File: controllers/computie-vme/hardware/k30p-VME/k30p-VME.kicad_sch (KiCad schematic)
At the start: 8 parts, among them J1 5V, J2 5V

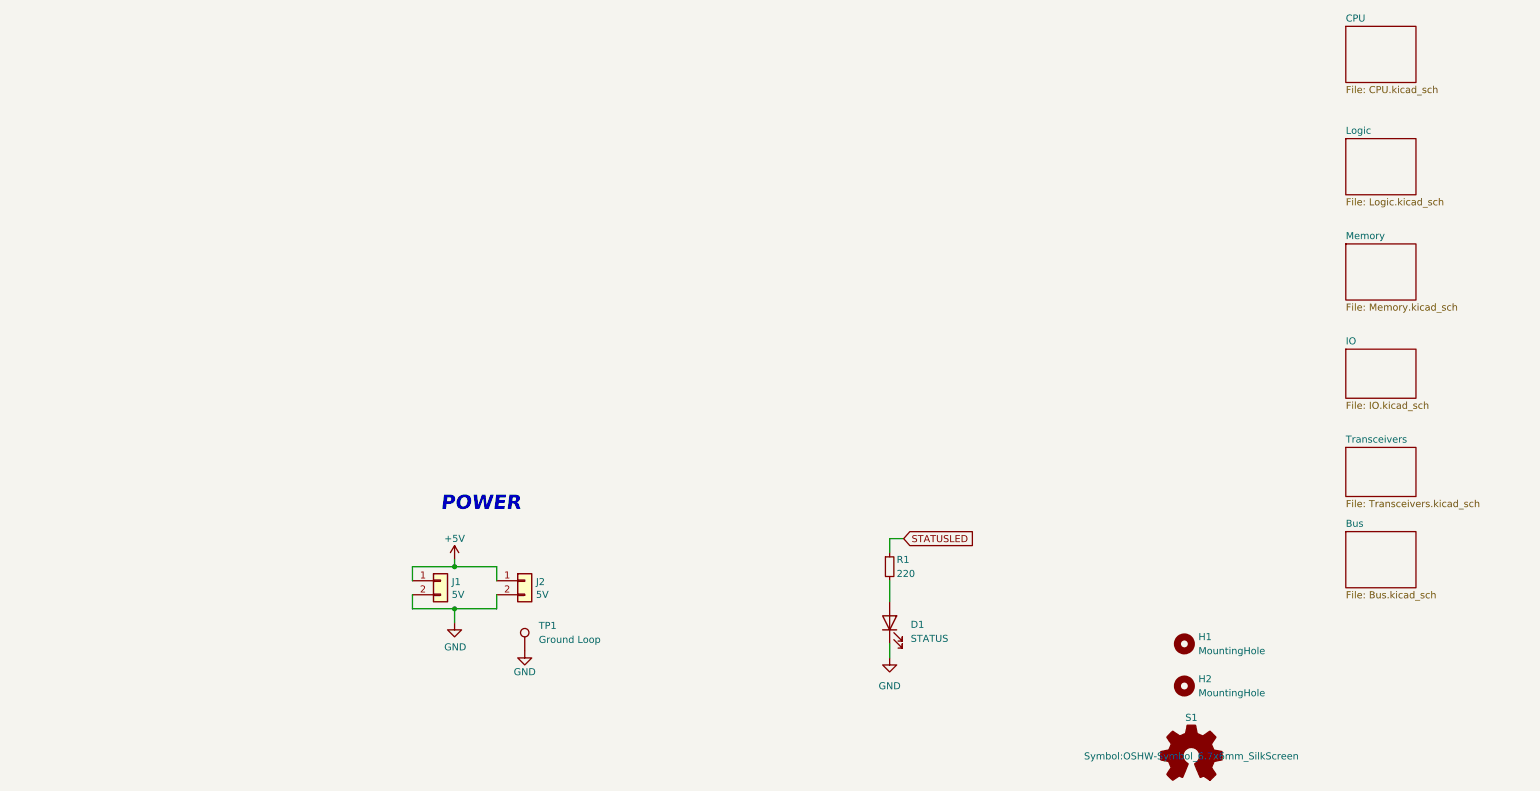
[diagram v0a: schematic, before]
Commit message: Updating with more work in progress
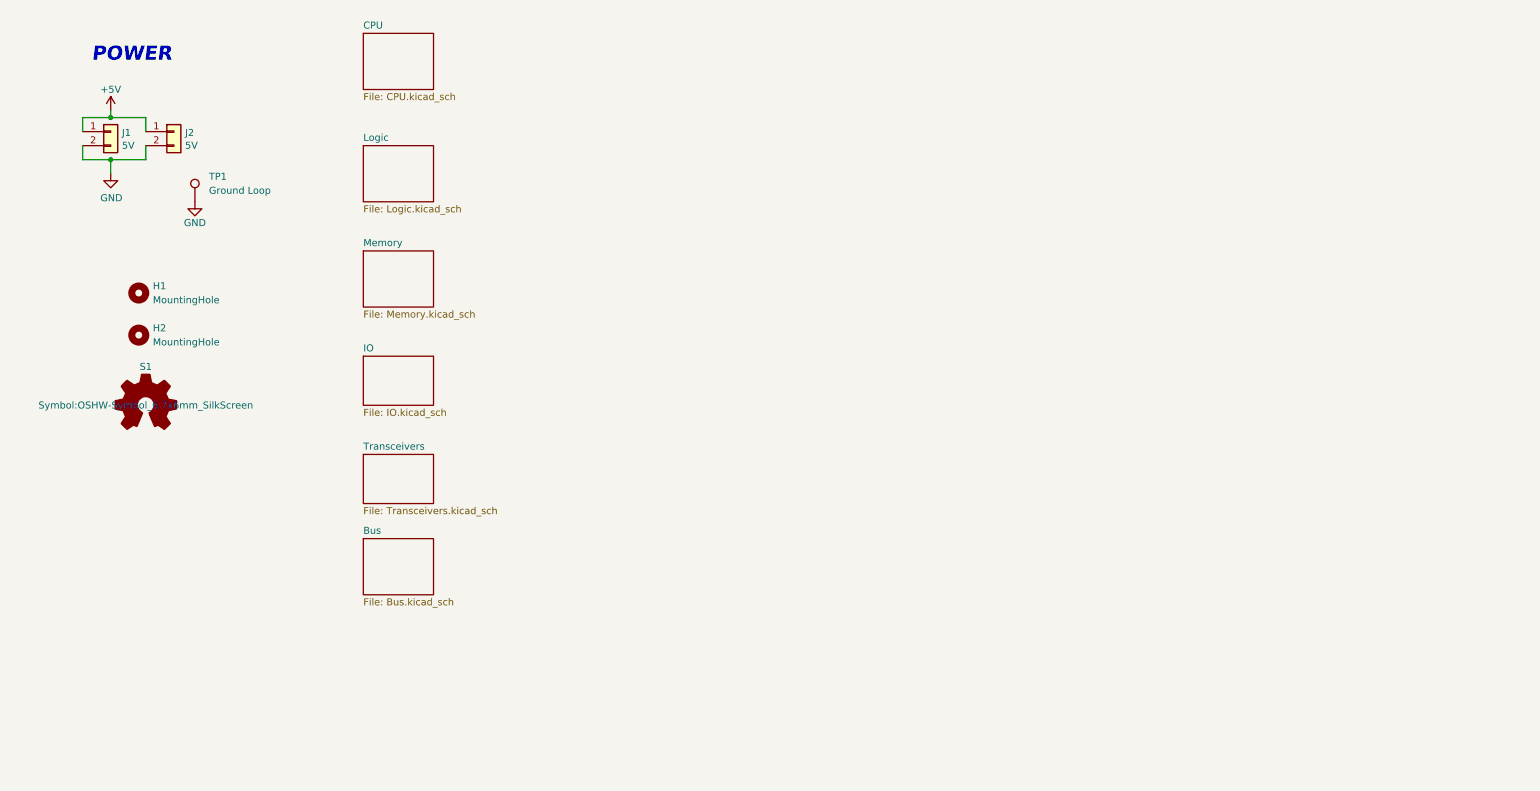
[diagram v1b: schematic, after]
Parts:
- removed D1: STATUS, LED_THT:LED_D3.0mm, symbol Device:LED
- removed R1: 220, Resistor_SMD:R_0805_2012Metric_Pad1.20x1.40mm_HandSolder, symbol Device:R_Small
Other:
- title: k30-VME32 -> k30p-VME
- moved on the sheet: H1, H2, J1, J2, S1, TP1

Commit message: Reorganized a bit
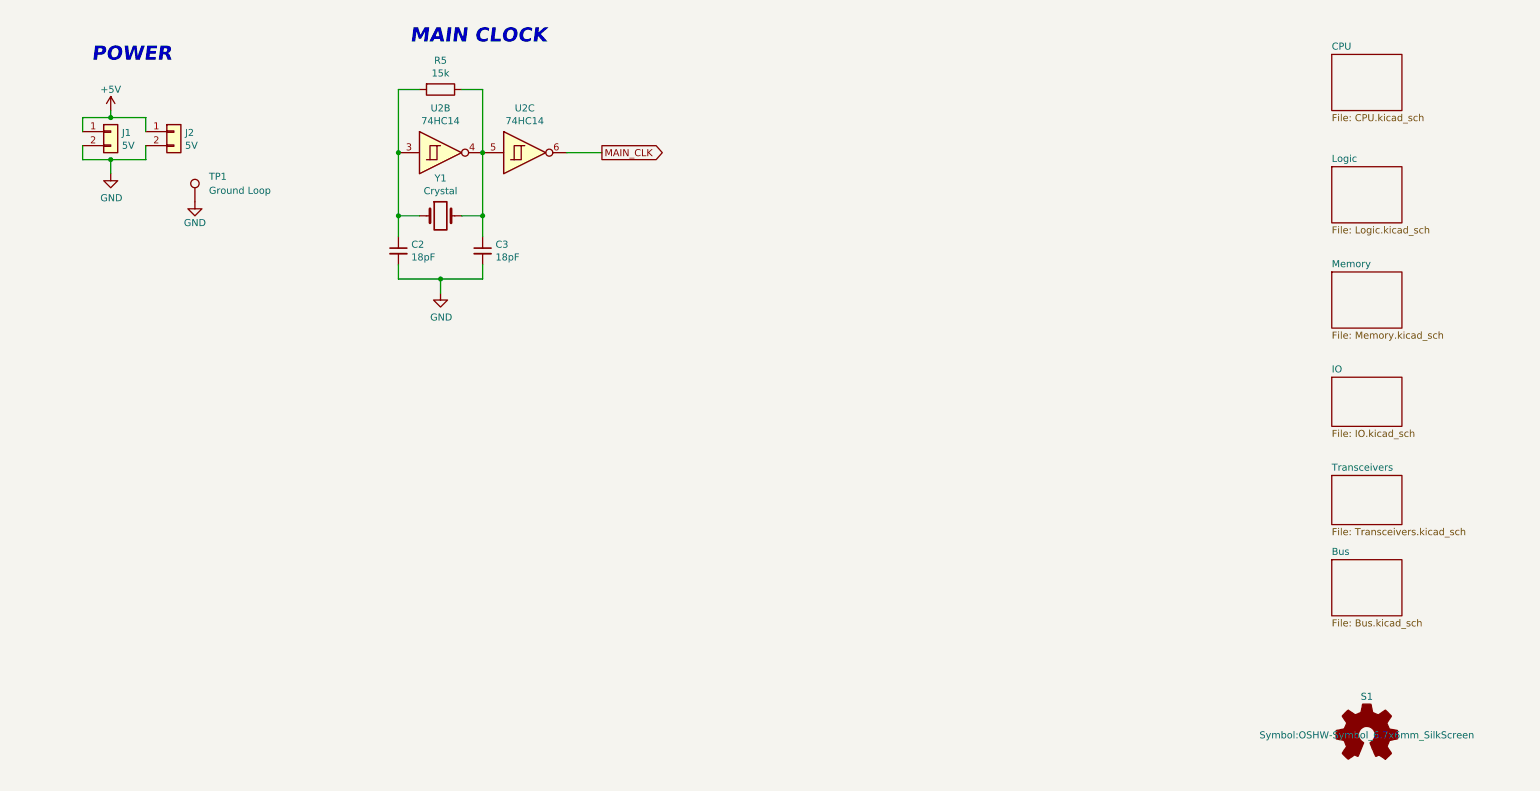
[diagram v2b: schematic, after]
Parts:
- removed H1, H2: MountingHole, MountingHole:MountingHole_2.7mm_M2.5_DIN965, symbol Mechanical:MountingHole
- added C2, C3: 18pF, Capacitor_THT:C_Disc_D3.0mm_W2.0mm_P2.50mm, symbol Device:C_Small
- added R5: 15k, Resistor_SMD:R_0805_2012Metric_Pad1.20x1.40mm_HandSolder, symbol Device:R
- added U2: 74HC14, Package_SO:TSSOP-14_4.4x5mm_P0.65mm, symbol 74xx:74HC14
- added Y1: Crystal, Crystal:Crystal_HC49-4H_Vertical, symbol Device:Crystal
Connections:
- net GND: now also C2.2, C3.2
- new net: C2.1, R5.2, U2.3, Y1.1
- new net: C3.1, R5.1, U2.4, U2.5, Y1.2
- new net MAIN_CLK: U2.6
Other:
- note added: "MAIN CLOCK"
- moved on the sheet: S1
